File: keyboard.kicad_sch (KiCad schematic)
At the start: 24 parts, among them SW1 SW_Push, U1 ATmega32U4-A, Y1 16MHz

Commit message: f
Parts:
- C1, C2, C3, C4, C5, C6, C7: footprint (none) -> Capacitor_SMD:C_0805_2012Metric
- D1, D2, D3, D4: footprint (none) -> Diode_SMD:D_SOD-123
- F1: footprint (none) -> Fuse:Fuse_1206_3216Metric
- MX1, MX2, MX3, MX4: footprint (none) -> MX_Only:MXOnly-1U-NoLED
- R1, R2, R3, R4: footprint (none) -> Resistor_SMD:R_0805_2012Metric
- SW1: footprint (none) -> random-keyboard-parts:SKQG-1155865
- USB1: footprint (none) -> random-keyboard-parts:Molex-0548190589
- Y1: footprint (none) -> Crystal:Crystal_SMD_3225-4Pin_3.2x2.5mm

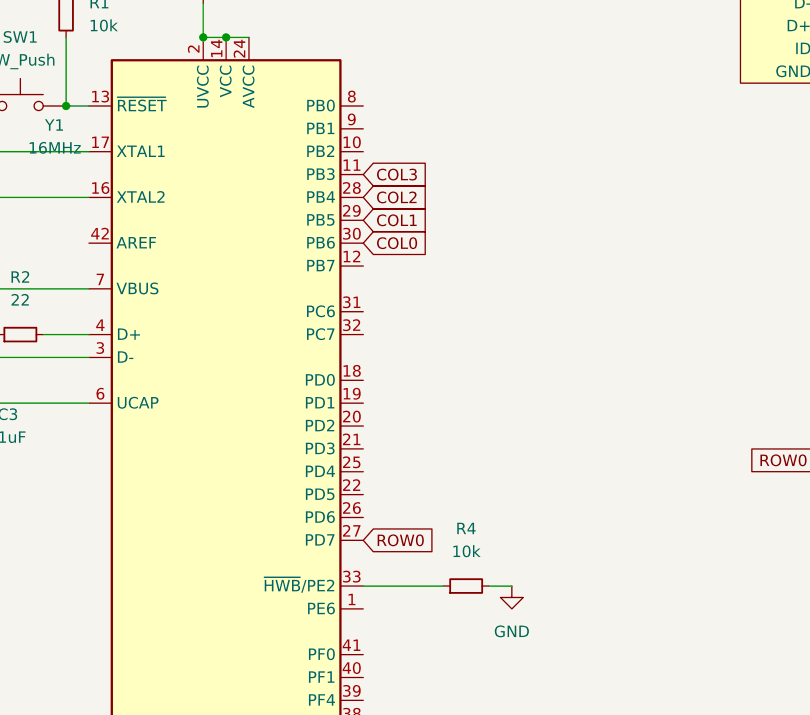
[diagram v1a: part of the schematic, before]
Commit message: e
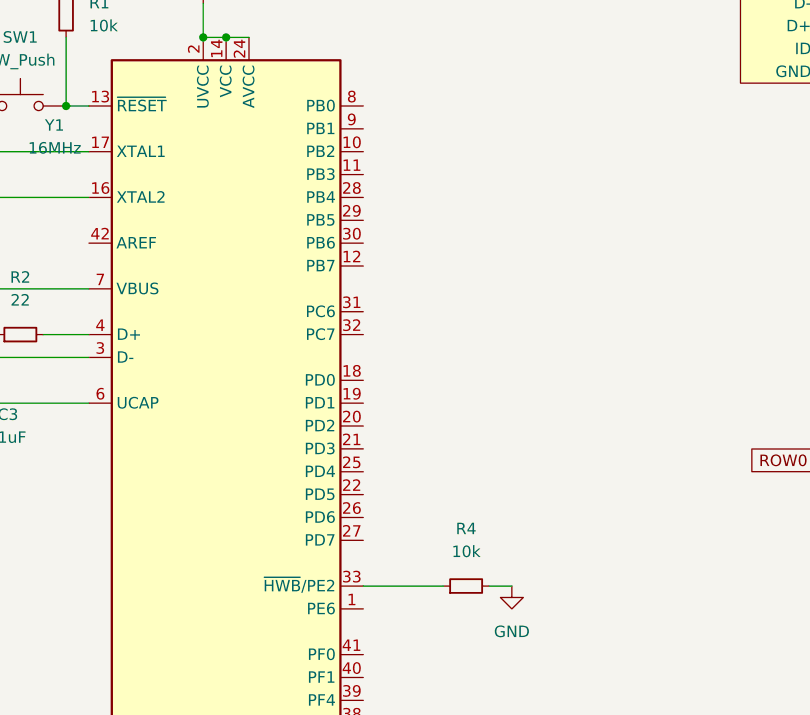
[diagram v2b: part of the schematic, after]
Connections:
- net COL0: no longer U1.30 (PB6)
- net COL1: no longer U1.29 (PB5)
- net COL2: no longer U1.28 (PB4)
- net COL3: no longer U1.11 (PB3)
- net ROW0: no longer U1.27 (PD7)
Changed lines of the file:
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@@
     (stroke (width 0) (type default) (color 0 0 0 0))
-  )
-  (global_label "ROW0" (shape input) (at 127 120.65 0) (fields_autoplaced)
-    (effects (font (size 1.27 1.27)) (justify left))
-    (property "Intersheet References" "${INTERSHEET_REFS}" (id 0) (at 134.6745 120.5706 0)
-      (effects (font (size 1.27 1.27)) (justify left) hide)
-    )
   )
   (global_label "D-" (shape input) (at 73.66 100.33 180) (fields_autoplaced)
@@
     )
   )
-  (global_label "COL2" (shape input) (at 127 82.55 0) (fields_autoplaced)
-    (effects (font (size 1.27 1.27)) (justify left))
-    (property "Intersheet References" "${INTERSHEET_REFS}" (id 0) (at 134.2512 82.4706 0)
-      (effects (font (size 1.27 1.27)) (justify left) hide)
-    )
-  )
   (global_label "COL1" (shape input) (at 208.28 88.9 90) (fields_autoplaced)
     (effects (font (size 1.27 1.27)) (justify left))
     (property "Intersheet References" "${INTERSHEET_REFS}" (id 0) (at 208.2006 81.6488 90)
-      (effects (font (size 1.27 1.27)) (justify left) hide)
-    )
-  )
-  (global_label "COL0" (shape input) (at 127 87.63 0) (fields_autoplaced)
-    (effects (font (size 1.27 1.27)) (justify left))
-    (property "Intersheet References" "${INTERSHEET_REFS}" (id 0) (at 134.2512 87.5506 0)
       (effects (font (size 1.27 1.27)) (justify left) hide)
     )
@@
     )
   )
-  (global_label "COL3" (shape input) (at 127 80.01 0) (fields_autoplaced)
-    (effects (font (size 1.27 1.27)) (justify left))
-    (property "Intersheet References" "${INTERSHEET_REFS}" (id 0) (at 134.2512 79.9306 0)
-      (effects (font (size 1.27 1.27)) (justify left) hide)
-    )
-  )
   (global_label "D-" (shape input) (at 182.88 60.96 0) (fields_autoplaced)
     (effects (font (size 1.27 1.27)) (justify left))
@@
       (effects (font (size 1.27 1.27)) (justify left) hide)
     )
-  )
-  (global_label "COL1" (shape input) (at 127 85.09 0) (fields_autoplaced)
-    (effects (font (size 1.27 1.27)) (justify left))
-    (property "Intersheet References" "${INTERSHEET_REFS}" (id 0) (at 134.2512 85.0106 0)
-      (effects (font (size 1.27 1.27)) (justify left) hide)
-    )

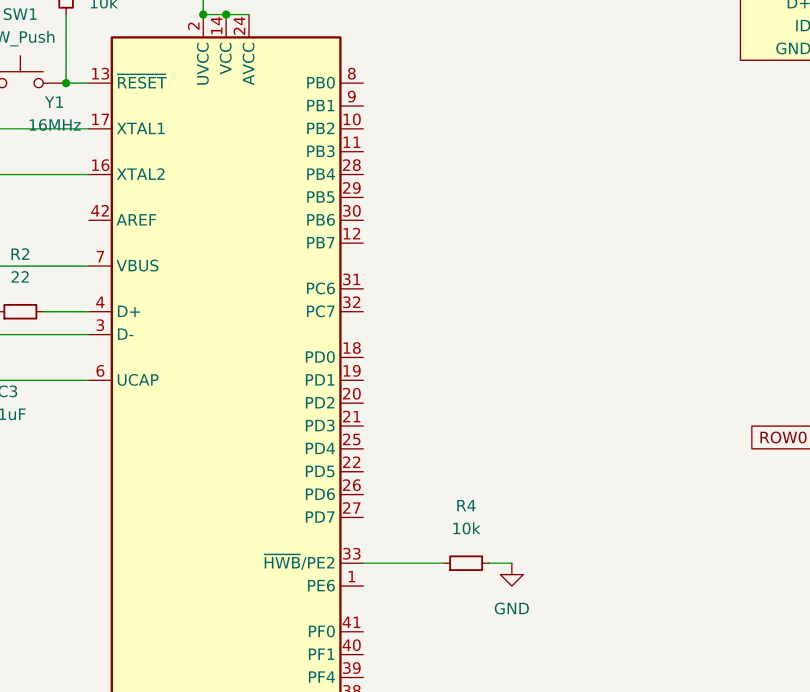
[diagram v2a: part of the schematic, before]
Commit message: k
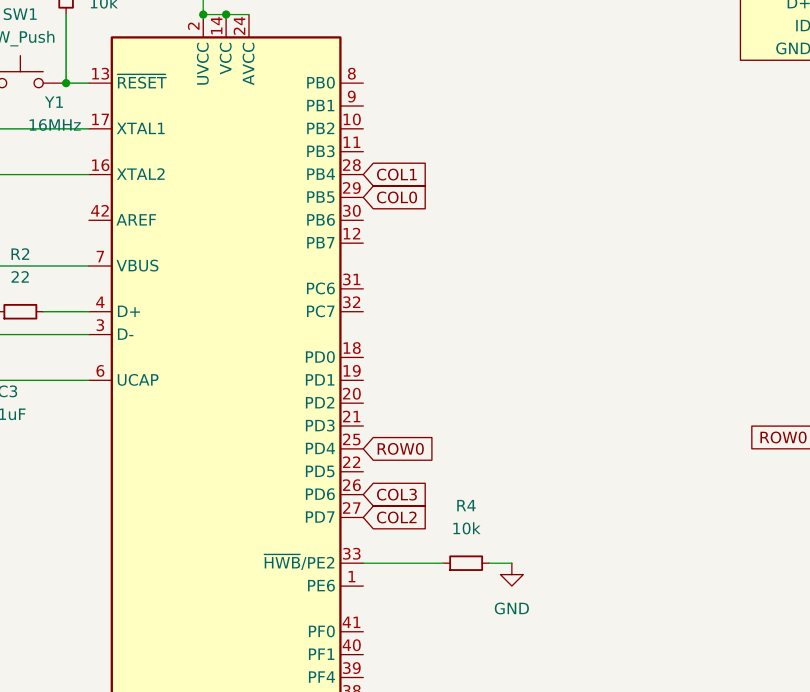
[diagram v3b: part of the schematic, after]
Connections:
- net COL0: now also U1.29 (PB5)
- net COL1: now also U1.28 (PB4)
- net COL2: now also U1.27 (PD7)
- net COL3: now also U1.26 (PD6)
- net ROW0: now also U1.25 (PD4)
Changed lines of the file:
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@@
     (stroke (width 0) (type default) (color 0 0 0 0))
+  )
+  (global_label "COL1" (shape input) (at 127 82.55 0) (fields_autoplaced)
+    (effects (font (size 1.27 1.27)) (justify left))
+    (property "Intersheet References" "${INTERSHEET_REFS}" (id 0) (at 134.2512 82.4706 0)
+      (effects (font (size 1.27 1.27)) (justify left) hide)
+    )
   )
   (global_label "D-" (shape input) (at 73.66 100.33 180) (fields_autoplaced)
@@
     )
   )
+  (global_label "ROW0" (shape input) (at 127 113.03 0) (fields_autoplaced)
+    (effects (font (size 1.27 1.27)) (justify left))
+    (property "Intersheet References" "${INTERSHEET_REFS}" (id 0) (at 134.6745 112.9506 0)
+      (effects (font (size 1.27 1.27)) (justify left) hide)
+    )
+  )
+  (global_label "COL0" (shape input) (at 127 85.09 0) (fields_autoplaced)
+    (effects (font (size 1.27 1.27)) (justify left))
+    (property "Intersheet References" "${INTERSHEET_REFS}" (id 0) (at 134.2512 85.0106 0)
+      (effects (font (size 1.27 1.27)) (justify left) hide)
+    )
+  )
   (global_label "D+" (shape input) (at 73.66 97.79 180) (fields_autoplaced)
     (effects (font (size 1.27 1.27)) (justify right))
     (property "Intersheet References" "${INTERSHEET_REFS}" (id 0) (at 68.4045 97.7106 0)
       (effects (font (size 1.27 1.27)) (justify right) hide)
+    )
+  )
+  (global_label "COL2" (shape input) (at 127 120.65 0) (fields_autoplaced)
+    (effects (font (size 1.27 1.27)) (justify left))
+    (property "Intersheet References" "${INTERSHEET_REFS}" (id 0) (at 134.2512 120.5706 0)
+      (effects (font (size 1.27 1.27)) (justify left) hide)
     )
   )
@@
       (effects (font (size 1.27 1.27)) (justify left) hide)
     )
+  )
+  (global_label "COL3" (shape input) (at 127 118.11 0) (fields_autoplaced)
+    (effects (font (size 1.27 1.27)) (justify left))
+    (property "Intersheet References" "${INTERSHEET_REFS}" (id 0) (at 134.2512 118.0306 0)
+      (effects (font (size 1.27 1.27)) (justify left) hide)
+    )
